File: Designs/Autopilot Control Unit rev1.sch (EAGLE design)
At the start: 44 parts, among them J1 CONNECTOR_3__0.1"_INCH_TH, J10 CONNECTOR_3__0.1"_INCH_TH, J11 CONNECTOR_3__0.1"_INCH_TH, J12 CONNECTOR_3__0.1"_INCH_TH, J2 CONNECTOR_3__0.1"_INCH_TH, J3 CONNECTOR_3__0.1"_INCH_TH, J4 CONNECTOR_3__0.1"_INCH_TH, J5 CONNECTOR_3__0.1"_INCH_TH, J6 CONNECTOR_3__0.1"_INCH_TH, J7 CONNECTOR_3__0.1"_INCH_TH, J8 CONNECTOR_3__0.1"_INCH_TH, J9 CONNECTOR_3__0.1"_INCH_TH, Q1 TRANSISTOR_N_MOS__PMV15ENEA, Q2 TRANSISTOR_N_MOS__PMV15ENEA, Q3 TRANSISTOR_N_MOS__PMV15ENEA, Q4 TRANSISTOR_N_MOS__PMV15ENEA, Q5 TRANSISTOR_N_MOS__PMV15ENEA, Q6 TRANSISTOR_N_MOS__PMV15ENEA, U1 ICM-42605, U2 VOLTAGE_REGULATOR_SOT-23-5_5V

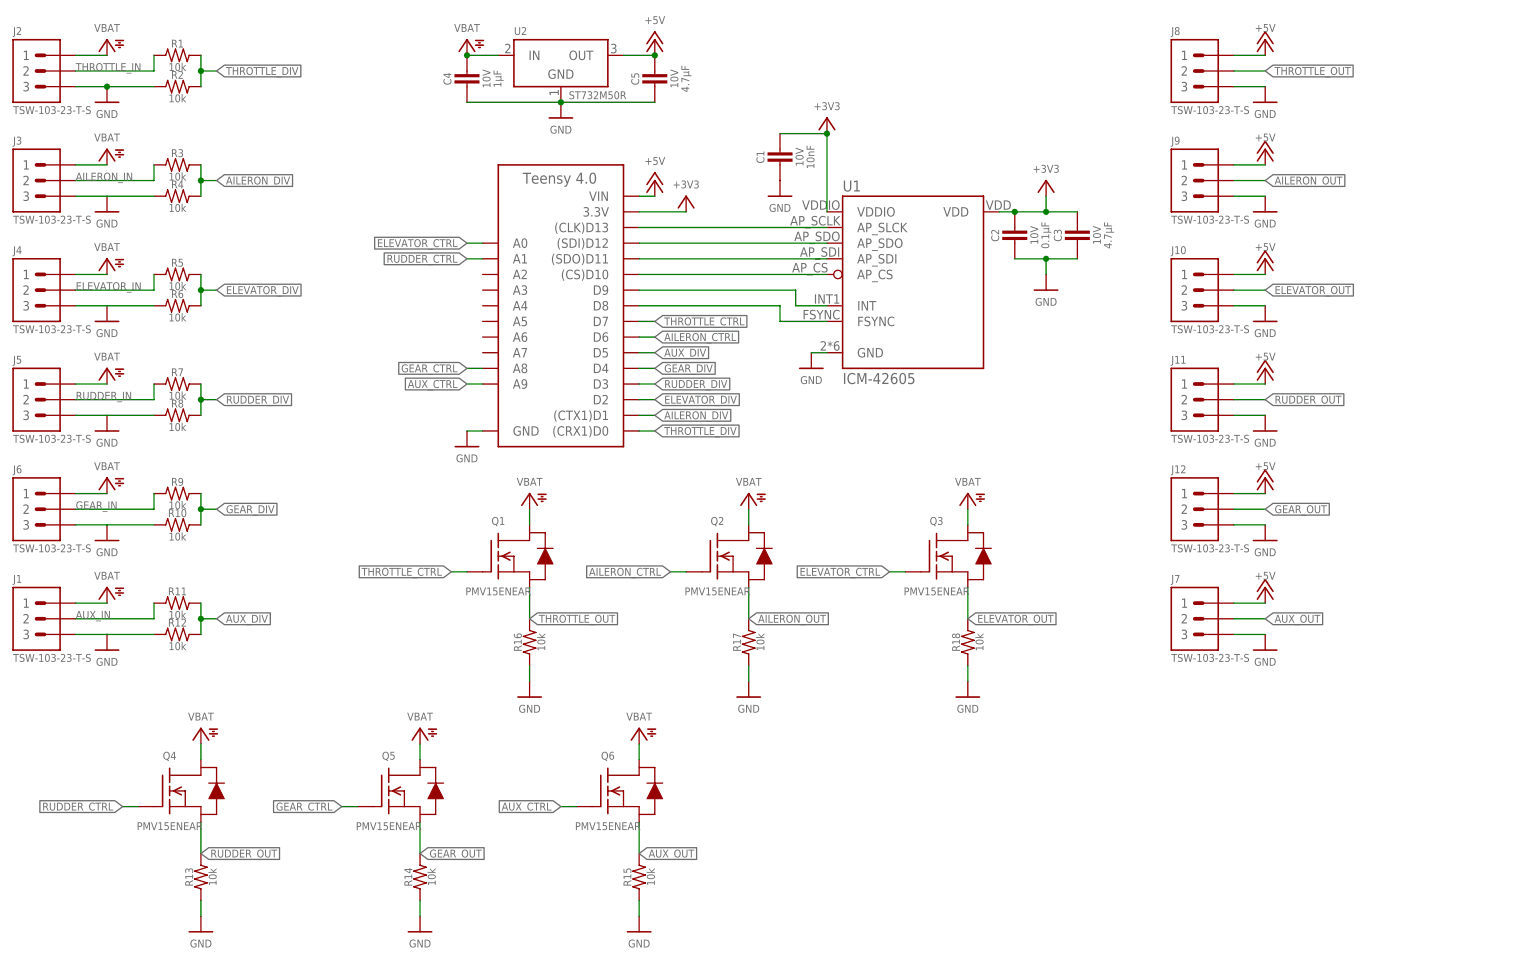
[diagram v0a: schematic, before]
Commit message: rev2
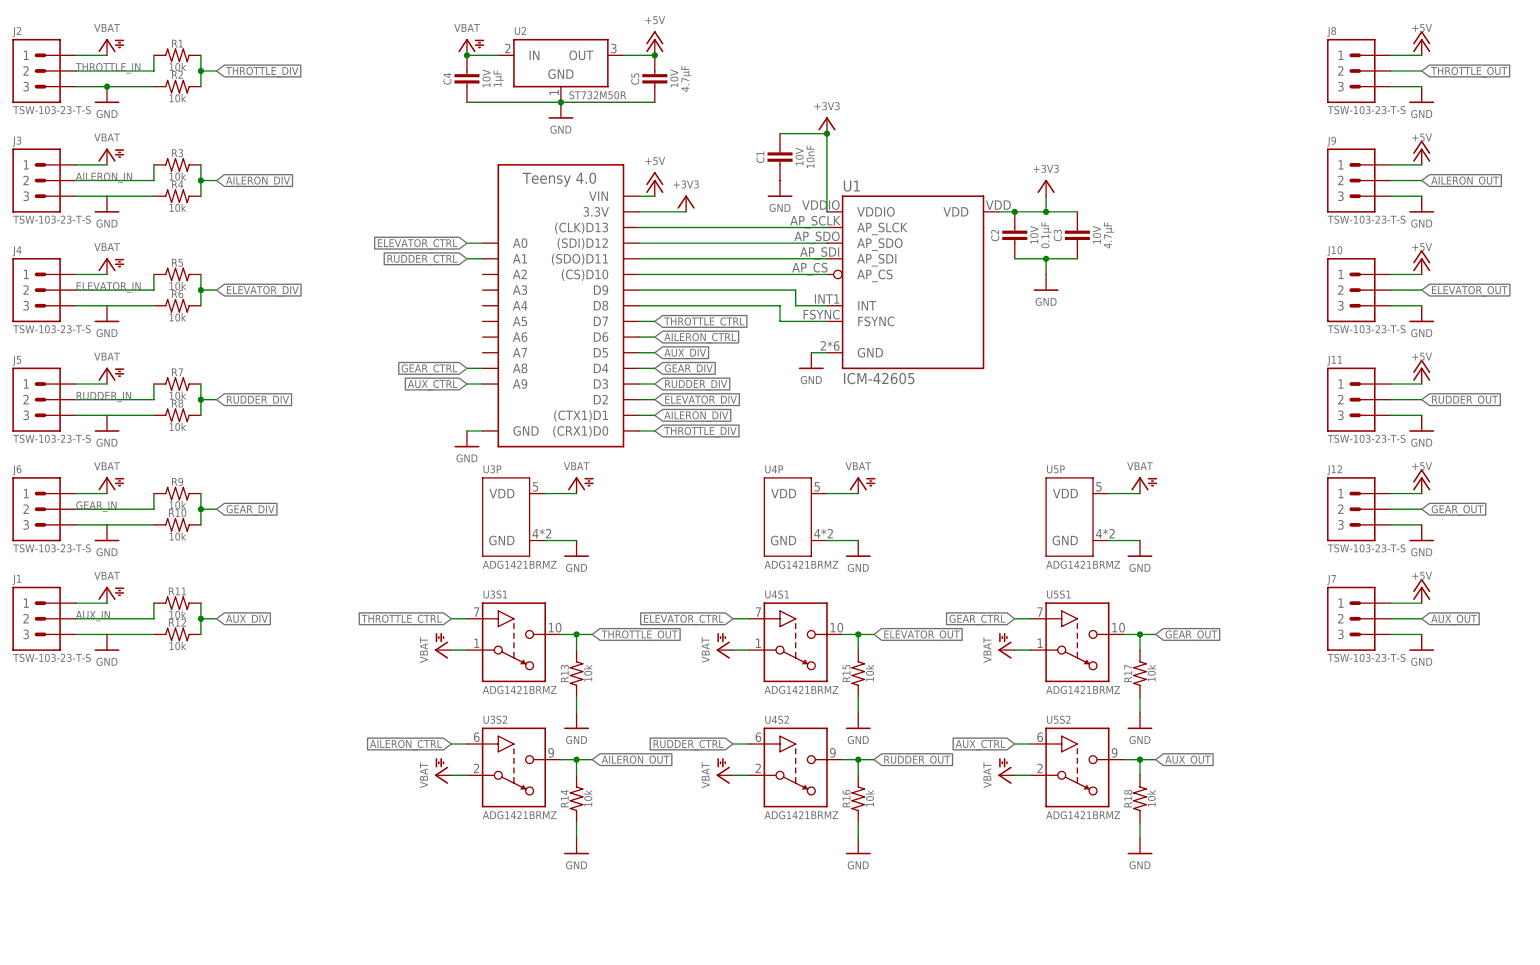
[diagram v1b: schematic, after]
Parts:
- removed Q1, Q2, Q3, Q4, Q5, Q6: TRANSISTOR_N_MOS__PMV15ENEA, HyTechDevices:TRANSISTOR_N_MOS__PMV15ENEA
- added U3, U4, U5: ADG1421, Devices:ADG1421
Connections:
- net AILERON_CTRL: now also U3S2.IN; no longer Q2.G
- net AILERON_OUT: now also R14.2, U3S2.D; no longer Q2.S, R17.2
- net AUX_CTRL: now also U5S2.IN; no longer Q6.G
- net AUX_OUT: now also R18.2, U5S2.D; no longer Q6.S, R15.2
- net ELEVATOR_CTRL: now also U4S1.IN; no longer Q3.G
- net ELEVATOR_OUT: now also R15.2, U4S1.D; no longer Q3.S, R18.2
- net GEAR_CTRL: now also U5S1.IN; no longer Q5.G
- net GEAR_OUT: now also R17.2, U5S1.D; no longer Q5.S, R14.2
- net GND: now also U3P.GND, U4P.GND, U5P.GND
- net RUDDER_CTRL: now also U4S2.IN; no longer Q4.G
- net RUDDER_OUT: now also R16.2, U4S2.D; no longer Q4.S, R13.2
- net THROTTLE_CTRL: now also U3S1.IN; no longer Q1.G
- net THROTTLE_OUT: now also R13.2, U3S1.D; no longer Q1.S, R16.2
- net VBAT: now also U3P.VDD, U3S1.S, U3S2.S, U4P.VDD, U4S1.S, U4S2.S, U5P.VDD, U5S1.S, U5S2.S; no longer Q1.D, Q2.D, Q3.D, Q4.D, Q5.D, Q6.D
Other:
- moved on the sheet: J10, J11, J12, J7, J8, J9, R13, R14, R15, R16, R17, R18
